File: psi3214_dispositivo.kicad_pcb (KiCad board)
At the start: 2 copper layers, 83 x 60.5 mm, 13 parts, among them J1 Screw_Terminal_01x02, J2 Screw_Terminal_01x03, U1 TL072_sim

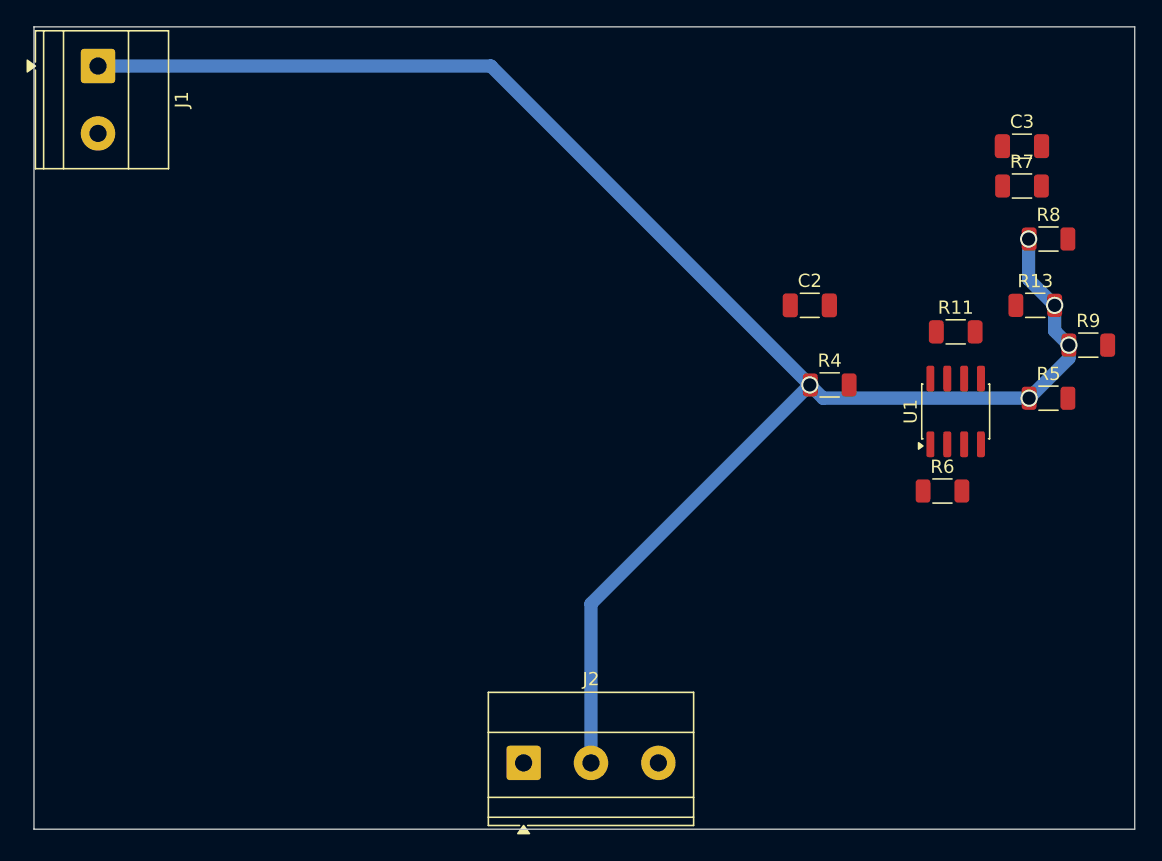
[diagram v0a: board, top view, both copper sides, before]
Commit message: PCB with ground plane version
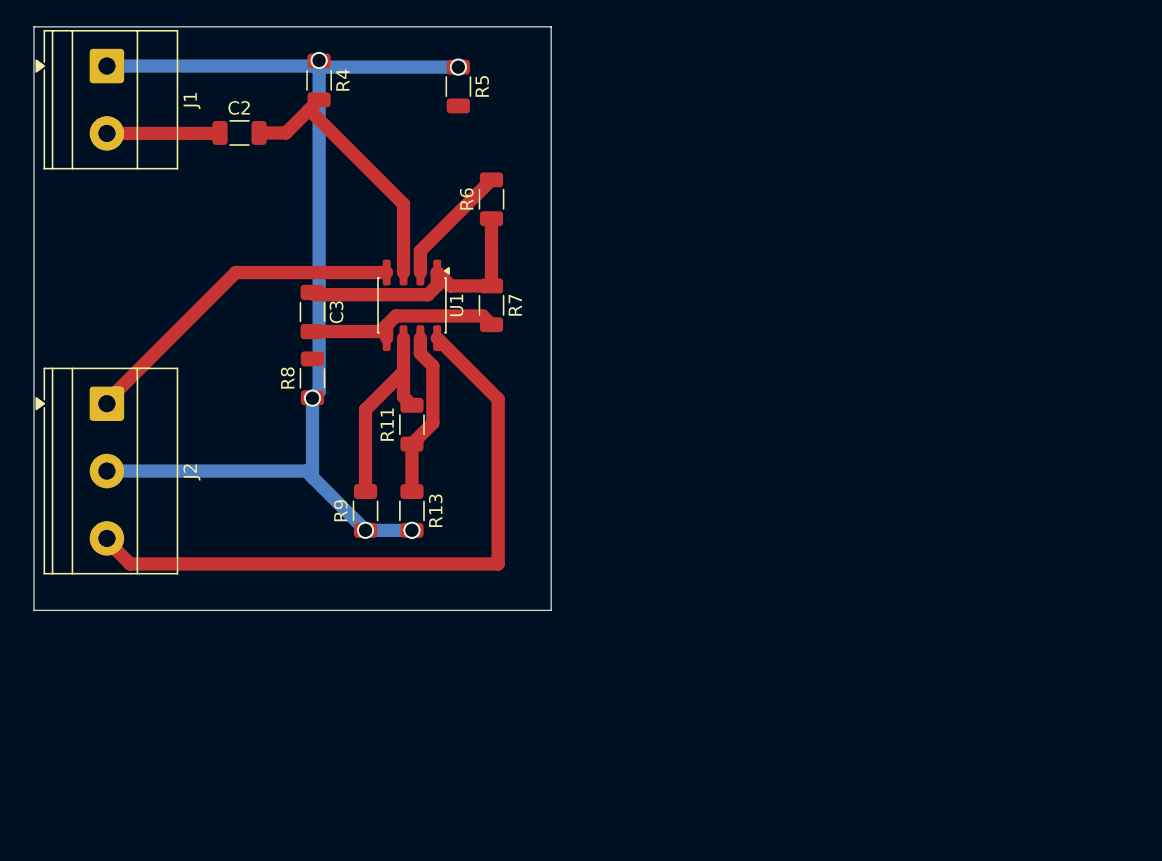
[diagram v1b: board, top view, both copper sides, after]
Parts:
- moved R8 56.5 mm to (155.5, 65.5), turned to 90 degrees
- moved R9 55.9 mm to (159.5, 75.5), turned to 90 degrees
- moved C3 54.9 mm to (155.5, 60.5), turned to -90 degrees
- moved R5 50.3 mm to (166.5, 43.5), turned to -90 degrees
- moved R13 49.5 mm to (163.0, 75.5), turned to -90 degrees
- moved C2 44.9 mm to (150.0, 47.0)
- moved R4 44.8 mm to (156.0, 43.0), turned to -90 degrees
- moved U1 41.8 mm to (163.0, 60.0), turned to -90 degrees
- moved R11 41.6 mm to (163.0, 69.0), turned to 90 degrees
- moved J2 41.5 mm to (140.0, 67.4), turned to -90 degrees
- moved R7 41.0 mm to (169.0, 60.0), turned to -90 degrees
- moved R6 40.5 mm to (169.0, 52.0), turned to 90 degrees
- moved J1 0.67 mm to (140.0, 42.0)
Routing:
- net +9V: track 0.00 -> 49.3 mm
- net GND: track 130.4 -> 83.4 mm
- net -9V: track 0.00 -> 25.3 mm
- net /saida_cap: track 0.00 -> 20.8 mm
- net /saida_amp1: track 0.00 -> 20.3 mm
- net Net-(U1B--): track 0.00 -> 15.5 mm
- net /saida_filtro: track 0.00 -> 15.2 mm
- net /saida: track 0.00 -> 12.6 mm
- net Net-(U1A--): track 0.00 -> 9.21 mm
- net /entrada: track 0.00 -> 8.54 mm
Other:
- board size 83 x 60.5 mm -> 39 x 44 mm
